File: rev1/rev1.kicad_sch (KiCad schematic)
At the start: 19 parts, among them J1 USB_C_Receptacle_USB2.0_14P, J2 P_IN, J3 DS3231, J4 Conn_02x15_Counter_Clockwise, M1 Left, M2 Right, Q1 MMBT5551L, Q2 MMBT5551L, U1 ESP32-S3-WROOM-1, U2 DS18B20

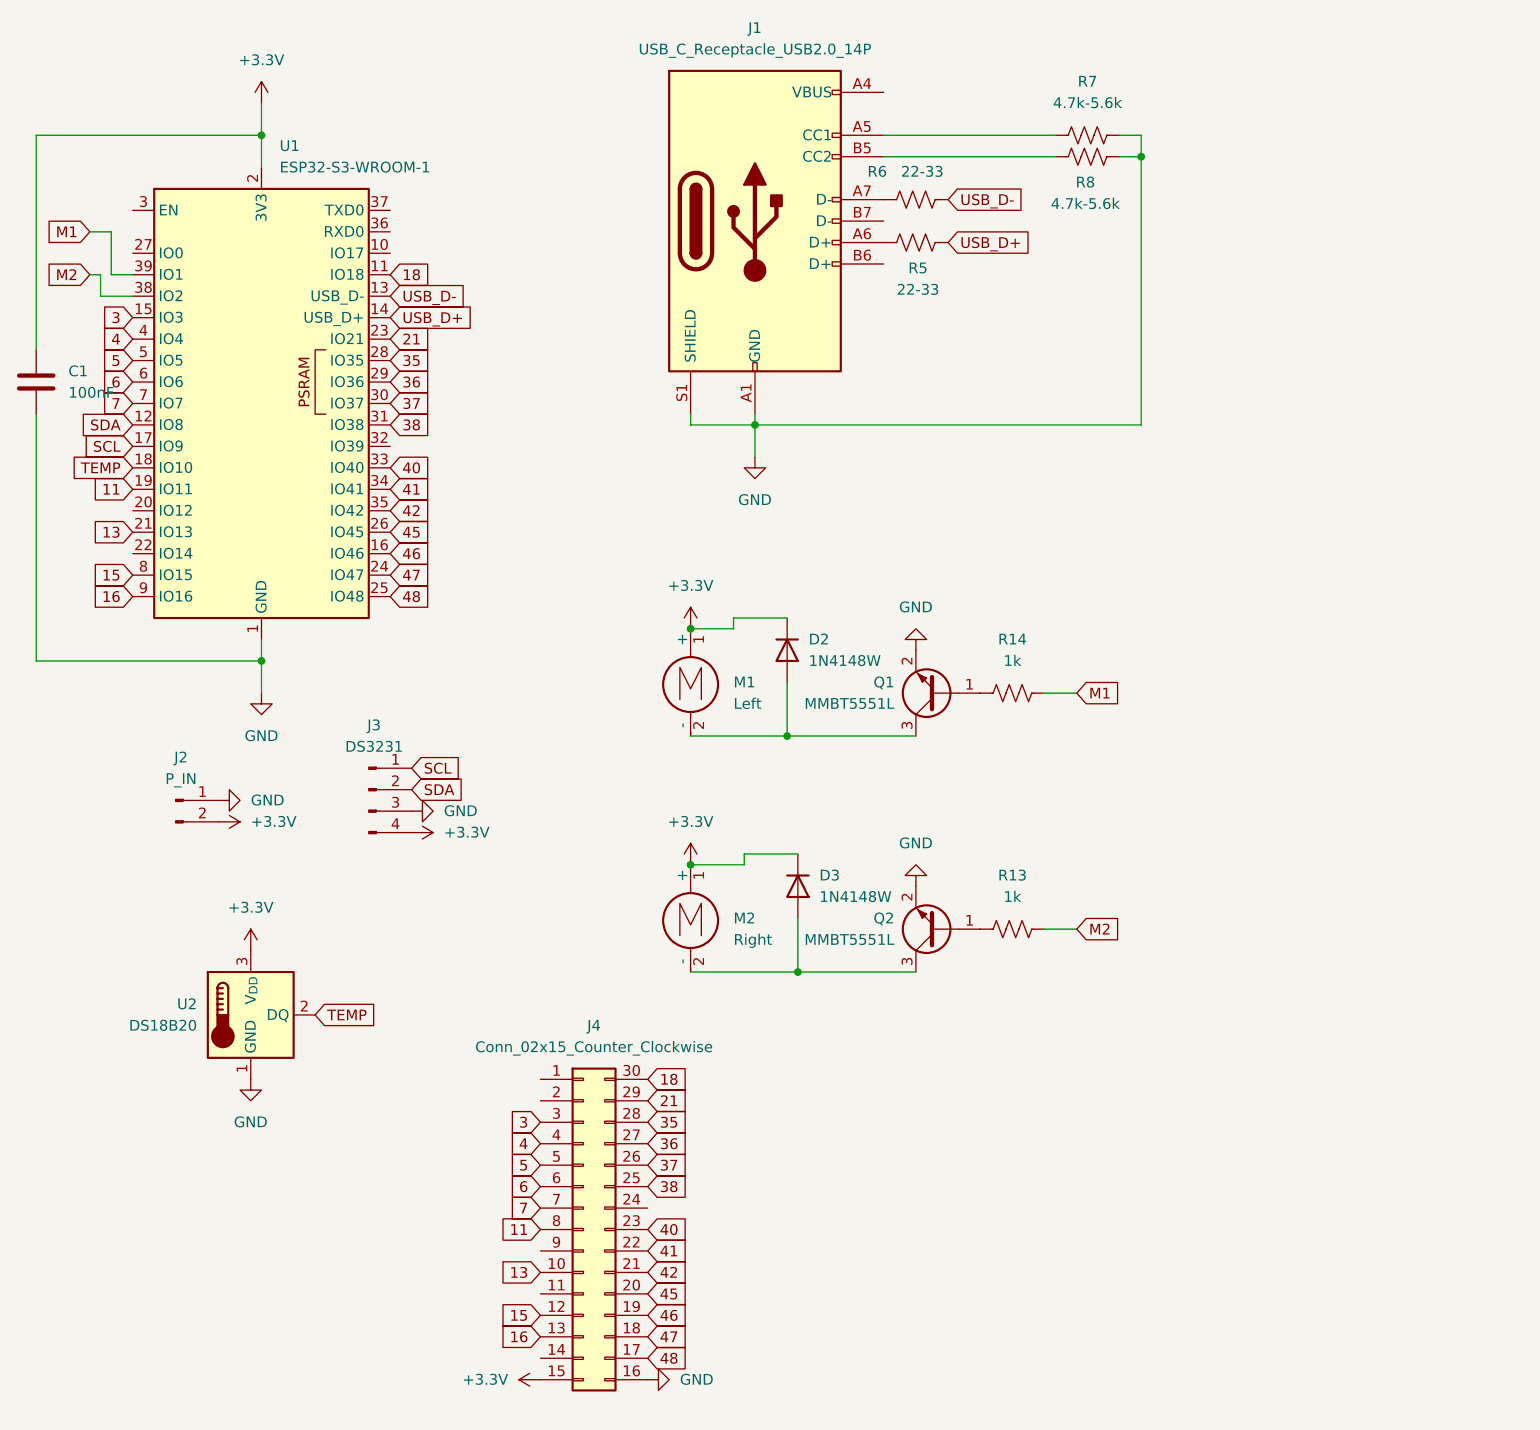
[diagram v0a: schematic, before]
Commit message: Schematic and PCB project
Made with KiCad 9.0
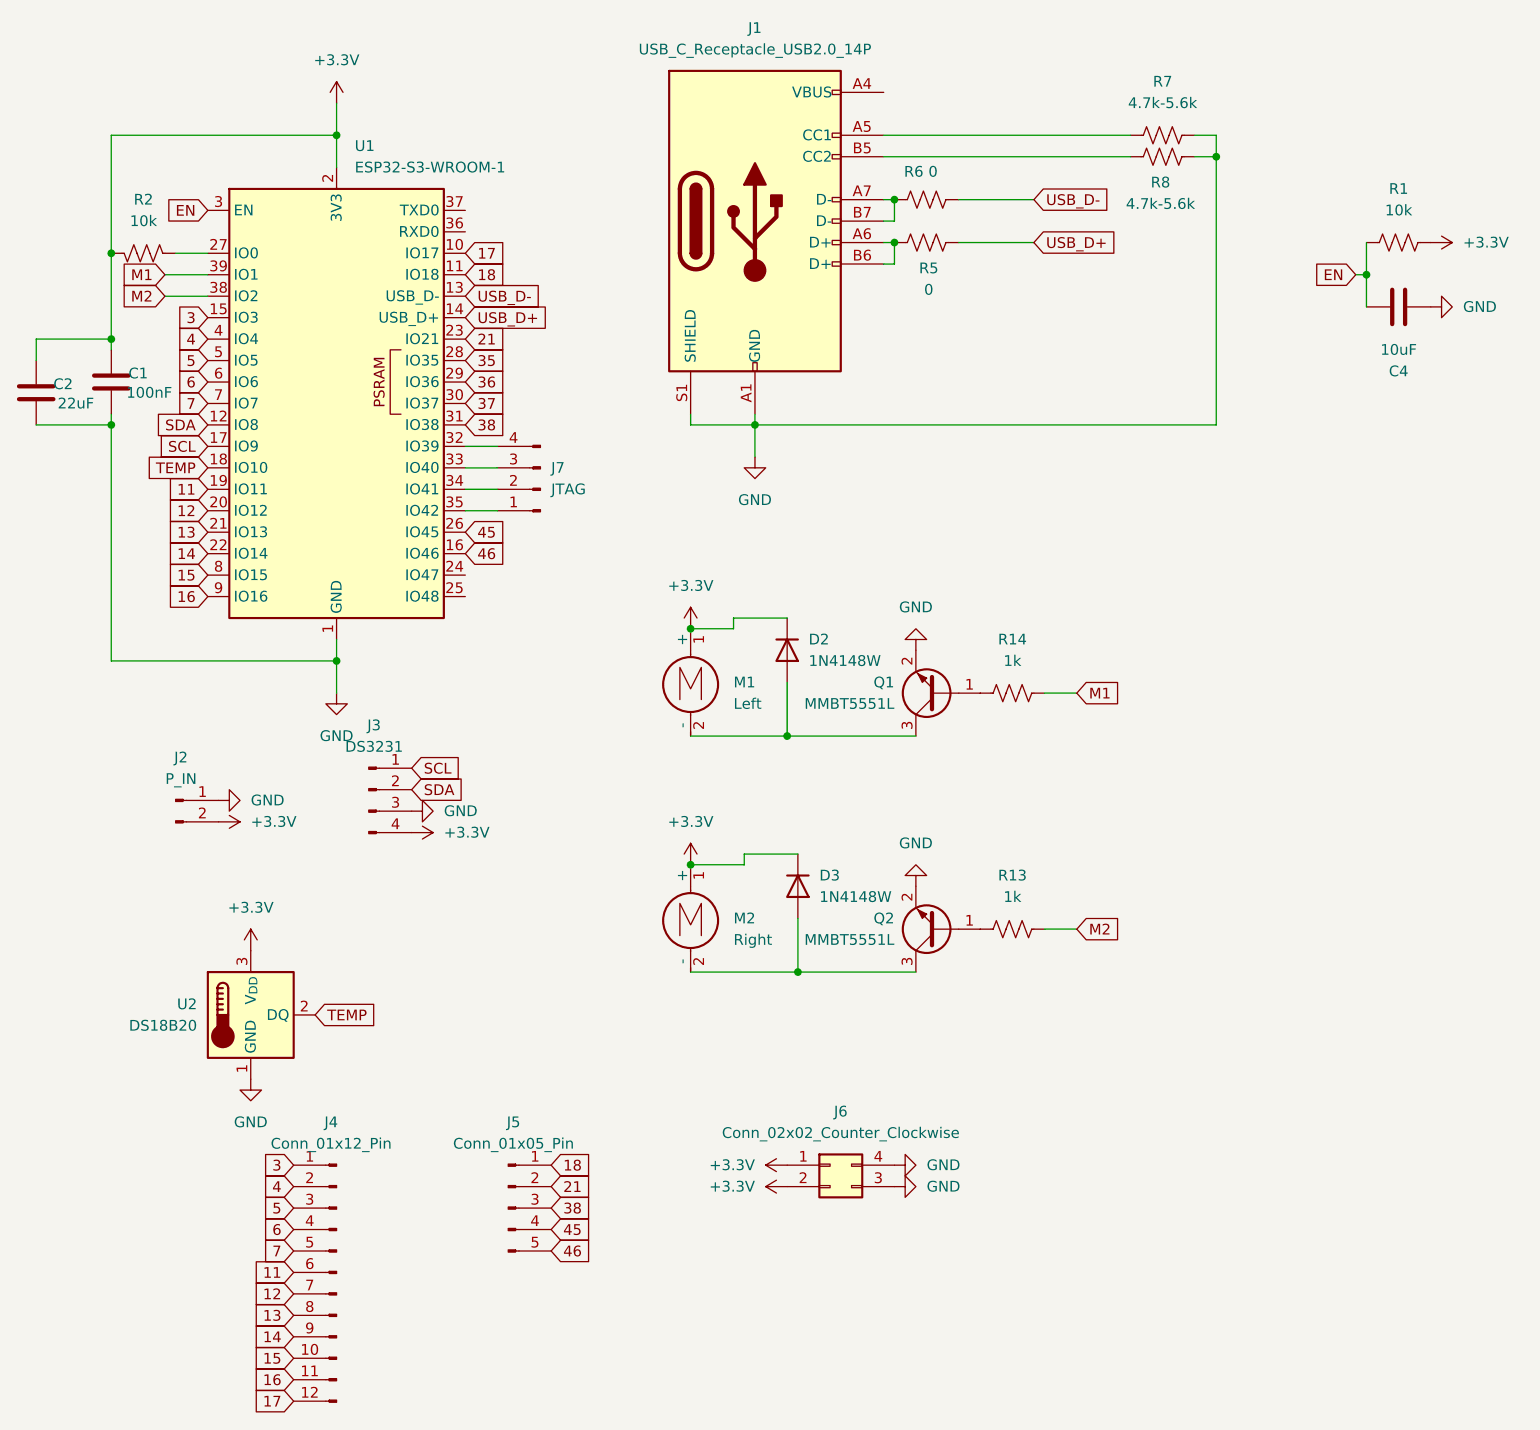
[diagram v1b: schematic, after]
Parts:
- removed J4: Conn_02x15_Counter_Clockwise, Connector_PinHeader_2.54mm:PinHeader_2x15_P2.54mm_Vertical, symbol Connector_Generic:Conn_02x15_Counter_Clockwise
- added C2: 22uF, Capacitor_SMD:C_0603_1608Metric_Pad1.08x0.95mm_HandSolder, symbol Device:C
- added C4: 10uF, Capacitor_SMD:C_0603_1608Metric_Pad1.08x0.95mm_HandSolder, symbol Device:C
- added J4: Conn_01x12_Pin, Connector_PinHeader_2.54mm:PinHeader_1x12_P2.54mm_Vertical, symbol Connector:Conn_01x12_Pin
- added J5: Conn_01x05_Pin, Connector_PinHeader_2.54mm:PinHeader_1x05_P2.54mm_Vertical, symbol Connector:Conn_01x05_Pin
- added J6: Conn_02x02_Counter_Clockwise, Connector_PinHeader_2.54mm:PinHeader_2x02_P2.54mm_Vertical, symbol Connector_Generic:Conn_02x02_Counter_Clockwise
- added J7: JTAG, Connector_PinHeader_2.54mm:PinHeader_1x04_P2.54mm_Vertical, symbol Connector:Conn_01x04_Pin
- added R1, R2: 10k, Resistor_SMD:R_0805_2012Metric_Pad1.20x1.40mm_HandSolder, symbol Device:R_US
- C1: footprint Capacitor_THT:CP_Radial_Tantal_D4.5mm_P5.00mm -> Capacitor_SMD:C_0603_1608Metric_Pad1.08x0.95mm_HandSolder
- R5, R6: value 22-33 -> 0
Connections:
- net +3.3V: now also C2.1, J6.1 (Pin_1), J6.2 (Pin_2), R1.2, R2.2
- net 11: now also J4.6 (Pin_6)
- net 13: now also J4.8 (Pin_8)
- net 15: now also J4.10 (Pin_10)
- net 16: now also J4.11 (Pin_11)
- net 18: now also J5.1 (Pin_1)
- net 21: now also J5.2 (Pin_2)
- net 3: now also J4.1 (Pin_1)
- net 38: now also J5.3 (Pin_3)
- net 4: now also J4.2 (Pin_2)
- net 45: now also J5.4 (Pin_4)
- net 46: now also J5.5 (Pin_5)
- net 5: now also J4.3 (Pin_3)
- net 6: now also J4.4 (Pin_4)
- net 7: now also J4.5 (Pin_5)
- net GND: now also C2.2, C4.1, J6.3 (Pin_3), J6.4 (Pin_4)
- net 17: now reaches U1.10 (IO17)
- net 17: now also J4.12 (Pin_12)
- net 12: now reaches U1.20 (IO12)
- net 12: now also J4.7 (Pin_7)
- net 14: now reaches U1.22 (IO14)
- net 14: now also J4.9 (Pin_9)
- net at U1.27 (IO0): now also R2.1
- net EN: now reaches U1.3 (EN)
- net EN: now also C4.2, R1.1
- net at U1.32 (IO39): now also J7.4 (Pin_4)
- net at J1.A6 (D+), R5.2: now also J1.B6 (D+)
- net at J1.A7 (D-), R6.2: now also J1.B7 (D-)
- net 40: no longer names the net of U1.33 (IO40)
- net 40: now also J7.3 (Pin_3)
- net 41: no longer names the net of U1.34 (IO41)
- net 41: now also J7.2 (Pin_2)
- net 42: no longer names the net of U1.35 (IO42)
- net 42: now also J7.1 (Pin_1)
- net 47: no longer names the net of U1.24 (IO47)
- net 48: no longer names the net of U1.25 (IO48)
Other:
- moved on the sheet: C1, R5, R6, R7, R8, U1
